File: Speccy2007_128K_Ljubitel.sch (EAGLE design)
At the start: 99 parts, among them X2 SCART-F, X5 ByteBlaster, X6 AVRISP

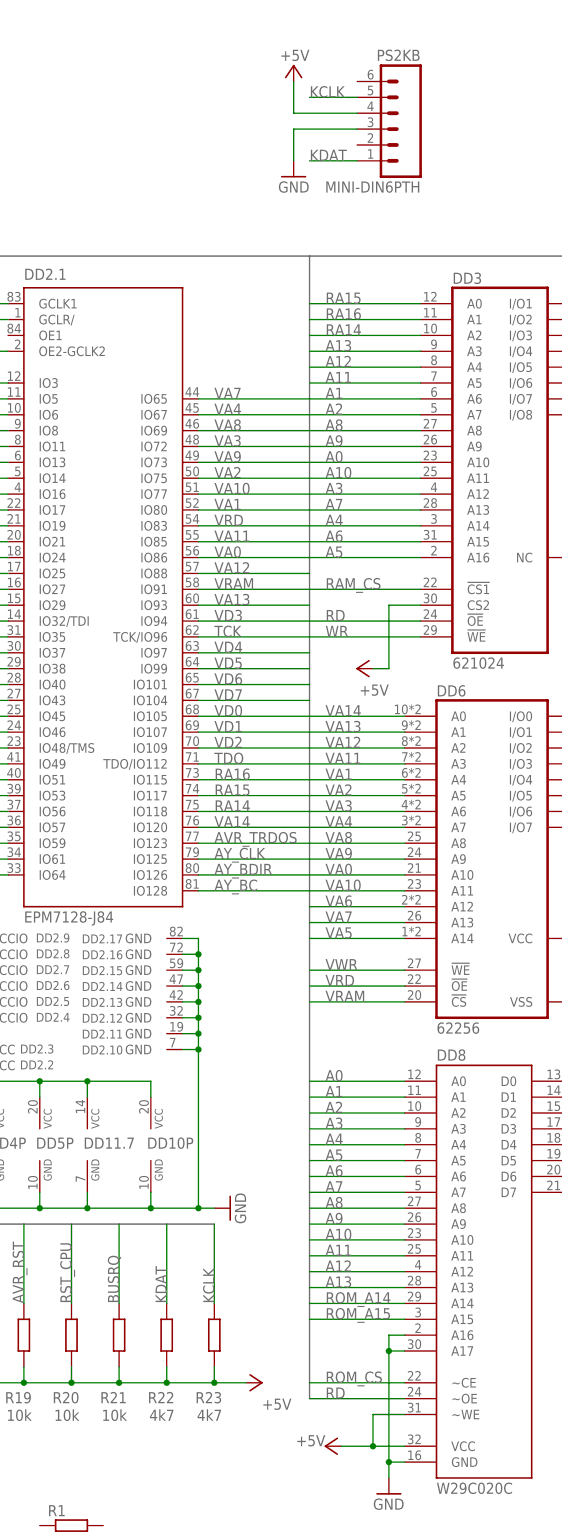
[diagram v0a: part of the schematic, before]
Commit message: .
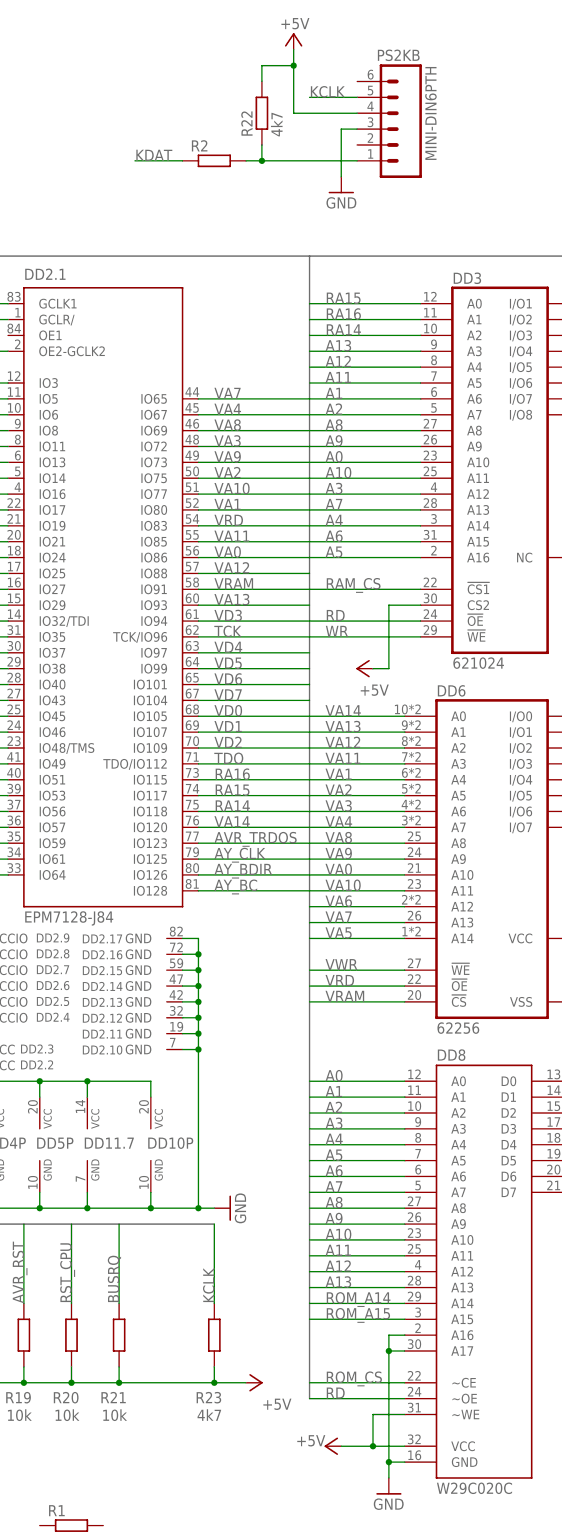
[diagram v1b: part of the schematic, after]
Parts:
- added R2: (no value), rcl:R-EU_M1206
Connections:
- new net N$24: PS2KB.1, R2.2, R22.1
- net +5V: now also R22.2; no longer R22.1
- net KDAT: now also R2.1; no longer PS2KB.1, R22.2
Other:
- moved on the sheet: R22
